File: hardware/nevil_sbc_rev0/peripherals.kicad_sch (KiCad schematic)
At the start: 18 parts, among them U201 74AC04, U202 74AC139, U203 74AC08, U204 CY62256-70PC, U205 28C256, U206 ATtiny84-20P, U207 VIA0, U208 VIA1

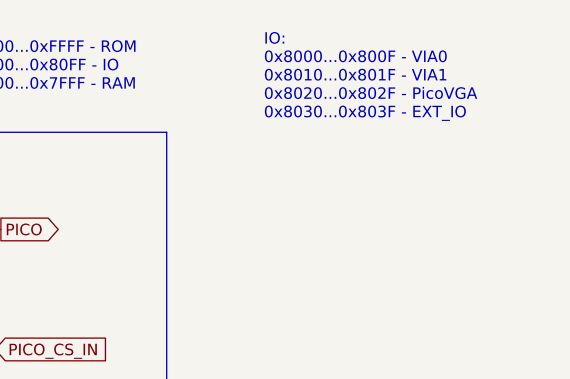
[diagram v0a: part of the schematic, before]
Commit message: working on vga code
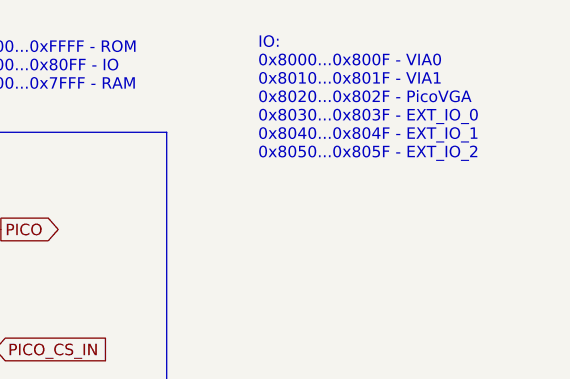
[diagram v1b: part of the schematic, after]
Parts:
- U202: footprint Package_SO:TSSOP-14_4.4x5mm_P0.65mm -> Package_SO:TSSOP-16_4.4x5mm_P0.65mm
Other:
- note added: "IO: 0x8000...0x800F - VIA0 0x8010...0x801F - VIA1 0x8020...0x802F - PicoVGA 0x8030...0x803F - EXT_IO_0 0x8040...0x804F - EXT_IO_1 0x8050...0x805F - EXT_IO_2"
- note removed: "IO: 0x8000...0x800F - VIA0 0x8010...0x801F - VIA1 0x8020...0x802F - PicoVGA 0x8030...0x803F - EXT_IO"
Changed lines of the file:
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@@
     (effects (font (size 1.27 1.27)) (justify left bottom))
   )
-  (text "IO:\n0x8000...0x800F - VIA0\n0x8010...0x801F - VIA1\n0x8020...0x802F - PicoVGA\n0x8030...0x803F - EXT_IO\n"
-    (at 256.54 23.495 0)
+  (text "IO:\n0x8000...0x800F - VIA0\n0x8010...0x801F - VIA1\n0x8020...0x802F - PicoVGA\n0x8030...0x803F - EXT_IO_0\n0x8040...0x804F - EXT_IO_1\n0x8050...0x805F - EXT_IO_2\n"
+    (at 255.905 27.94 0)
     (effects (font (size 1.27 1.27)) (justify left bottom))
   )
@@
     (property "Reference" "U202" (id 0) (at 144.78 40.005 0))
     (property "Value" "74AC139" (id 1) (at 144.78 42.545 0))
-    (property "Footprint" "Package_SO:TSSOP-14_4.4x5mm_P0.65mm" (id 2) (at 144.78 48.895 0)
+    (property "Footprint" "Package_SO:TSSOP-16_4.4x5mm_P0.65mm" (id 2) (at 144.78 48.895 0)
       (effects (font (size 1.27 1.27)) hide)
     )
@@
       (effects (font (size 1.27 1.27)) (justify left))
     )
-    (property "Footprint" "Package_SO:TSSOP-14_4.4x5mm_P0.65mm" (id 2) (at 83.82 36.83 0)
+    (property "Footprint" "Package_SO:TSSOP-16_4.4x5mm_P0.65mm" (id 2) (at 83.82 36.83 0)
       (effects (font (size 1.27 1.27)) hide)
     )
@@
     (property "Reference" "U202" (id 0) (at 145.415 17.78 0))
     (property "Value" "74AC139" (id 1) (at 144.78 20.32 0))
-    (property "Footprint" "Package_SO:TSSOP-14_4.4x5mm_P0.65mm" (id 2) (at 145.415 26.67 0)
-      (effects (font (size 1.27 1.27)) hide)
-    )
+    (property "Footprint" "Package_SO:TSSOP-16_4.4x5mm_P0.65mm" (id 2) (at 145.415 26.67 0)
+      (effects (font (size 1.27 1.27)) hide)
+    )
